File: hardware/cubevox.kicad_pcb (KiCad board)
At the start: 4 copper layers, 200 x 150 mm, 223 parts, among them J1 USB-C, J101 J_IN NCJ6FA-H, J106 DC 9V, J108 OUT 6.35mm, J117 OLED SH1106, J3 TC2030-NL SWD, K101 G6K-2F-Y DC5, K102 G6K-2F-Y DC5, Q101 MMBT3904, SW101 ST-0-102 bat toggle, SW102 ST-0-102 bat toggle, SW103 ST-0-102 bat toggle, SW104 ST-0-102 bat toggle, SW105 ST-0-102 bat toggle, SW106 ST-0-102 bat toggle, SW107 ST-0-102 bat toggle, SW108 ST-0-102 bat toggle, U1 STM32H743VIT6, U101 CD74HC4067, U103 AP63205WU-7, U104 OPA2197IDR, U105 OPA2197IDR, U106 OPA2197IDR, U3 AP63203WU-7, U4 TLV75533PDBVR, U6 PCM5102APWR, U8 PCM1808PWR, Y1 25MHz 12pF

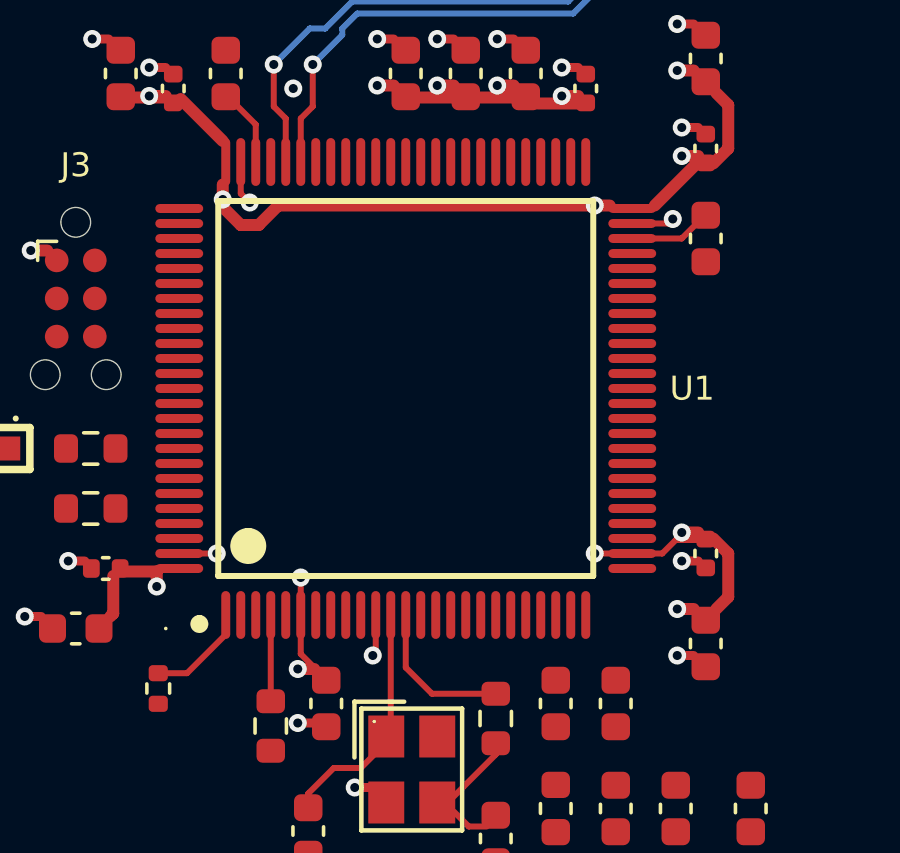
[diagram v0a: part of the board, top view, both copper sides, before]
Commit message: layout: change on /3V3,/GND (ledger 0098)
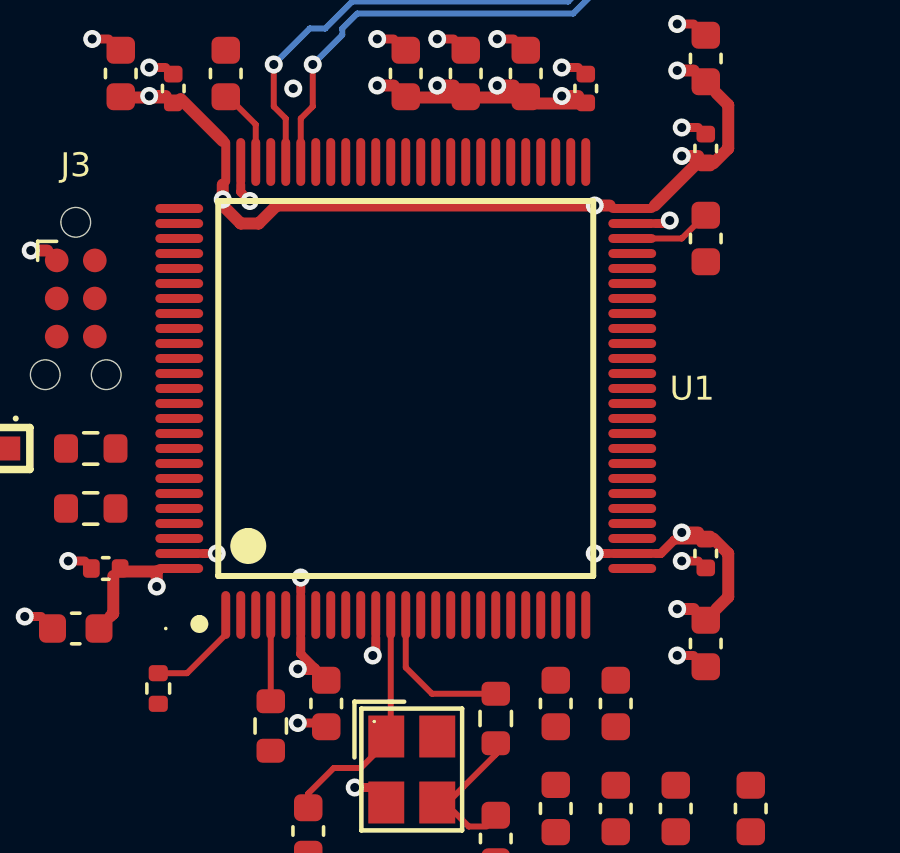
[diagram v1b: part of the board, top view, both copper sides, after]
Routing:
- net /3V3: track 610.6 -> 639.1 mm

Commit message: layout: change on /3V3 (ledger 0099)
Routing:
- net /3V3: track 639.1 -> 637.6 mm

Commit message: layout: change on /3V3 (ledger 0100)
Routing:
- net /3V3: track 637.6 -> 638.5 mm
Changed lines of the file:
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@@
+	)
+	(segment
+		(start 93.8 99.85)
+		(end 77.35 99.85)
+		(width 0.4)
+		(layer "In2.Cu")
+		(net "/3V3")
 	)
 	(segment
@@
 	)
 	(segment
-		(start 92.5 98.55)
-		(end 76.05 98.55)
-		(width 0.4)
-		(layer "In2.Cu")
-		(net "/3V3")
-	)
-	(segment
 		(start 124.7 101.95)
 		(end 125.25 102.5)
@@
 	)
 	(segment
-		(start 93.15 99.2)
-		(end 92.5 98.55)
+		(start 207.6 123.8)
+		(end 231.6 123.8)
 		(width 0.4)
 		(layer "In2.Cu")
@@
 	)
 	(segment
-		(start 207.6 123.8)
-		(end 231.6 123.8)
-		(width 0.4)
-		(layer "In2.Cu")
-		(net "/3V3")
-	)
-	(segment
 		(start 169.05 65.15)
 		(end 170 66.099999)
@@
 	)
 	(segment
+		(start 77.35 99.85)
+		(end 76.05 98.55)
+		(width 0.4)
+		(layer "In2.Cu")
+		(net "/3V3")
+	)
+	(segment
 		(start 112.15 62.75)
 		(end 117.25 62.75)
@@
 	)
 	(segment
+		(start 92.4 93.35)
+		(end 93.15 94.1)
+		(width 0.4)
+		(layer "In2.Cu")
+		(net "/3V3")
+	)
+	(segment
 		(start 83.5 79.4)
 		(end 82.55 80.35)
@@
 		(width 0.4)
 		(layer "In2.Cu")
-		(net "/3V3")
-	)
-	(segment
-		(start 92.4 93.35)
-		(end 93.15 94.1)
-		(width 0.4)
-		(layer "In2.Cu")
